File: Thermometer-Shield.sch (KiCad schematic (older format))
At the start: 33 parts, among them J1 CONN_01X04, J2 CONN_01X02, J3 CONN_01X02, J4 CONN_01X02, J5 CONN_01X02, SW1 SW_SPST, SW2 SW_SPST, SW3 SW_SPST, SW4 SW_SPST, U1 ULN2803A

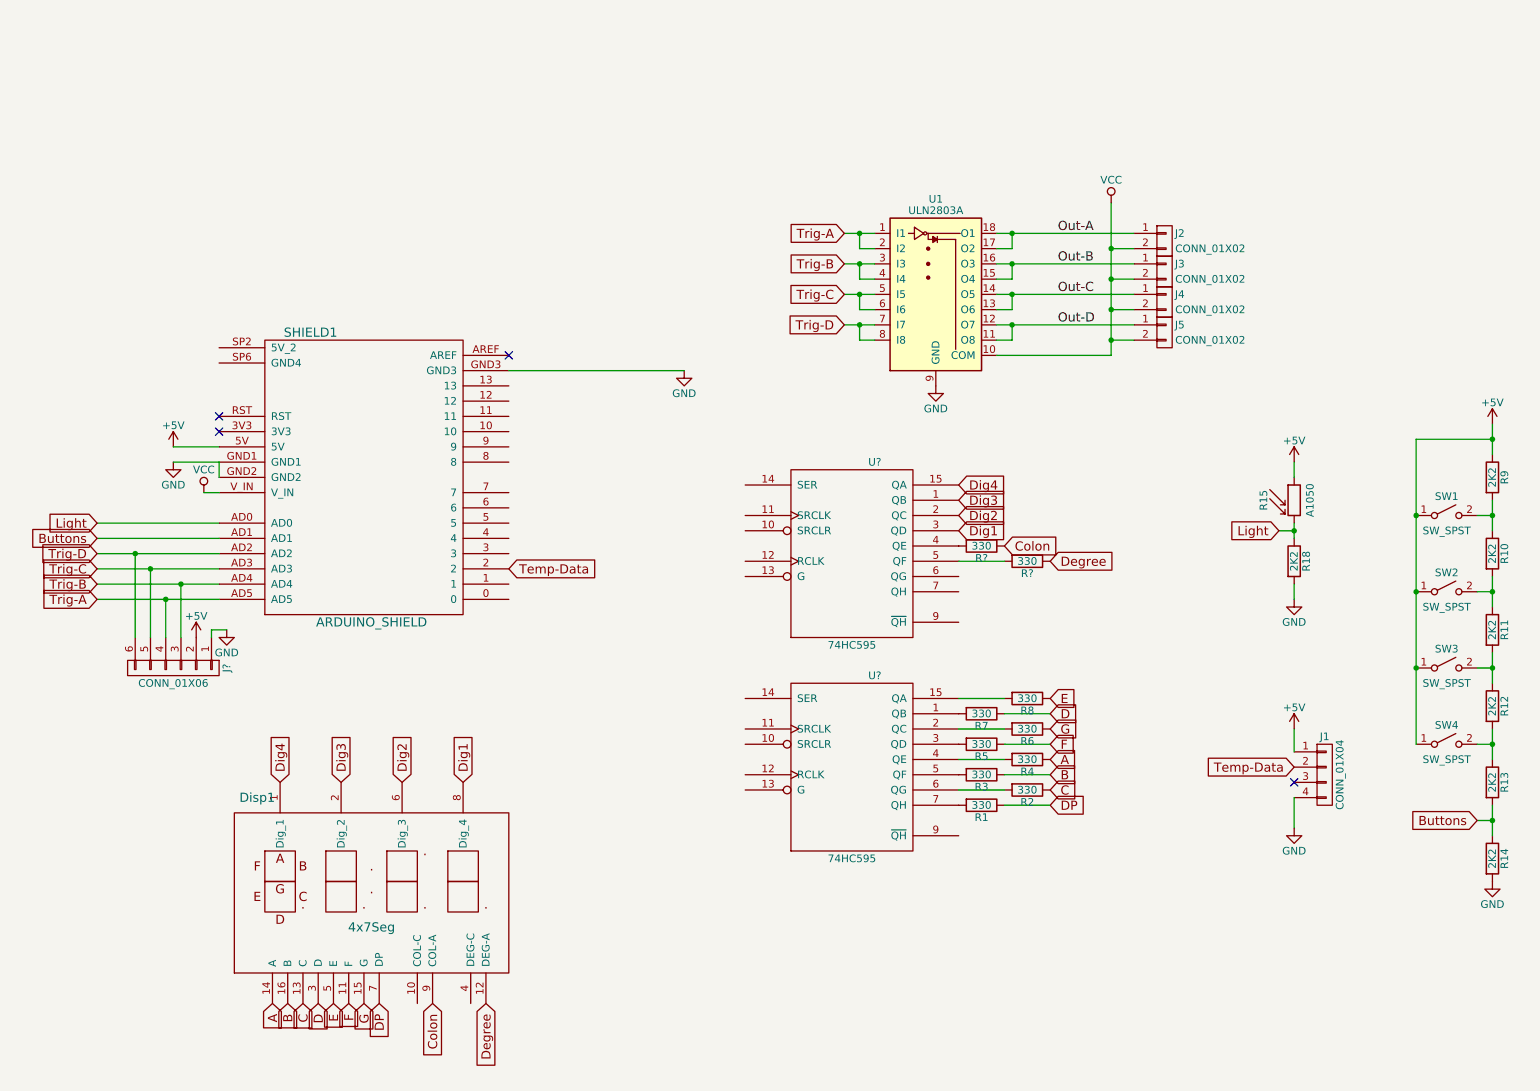
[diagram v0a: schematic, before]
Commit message: schematic nearly done. PCB started
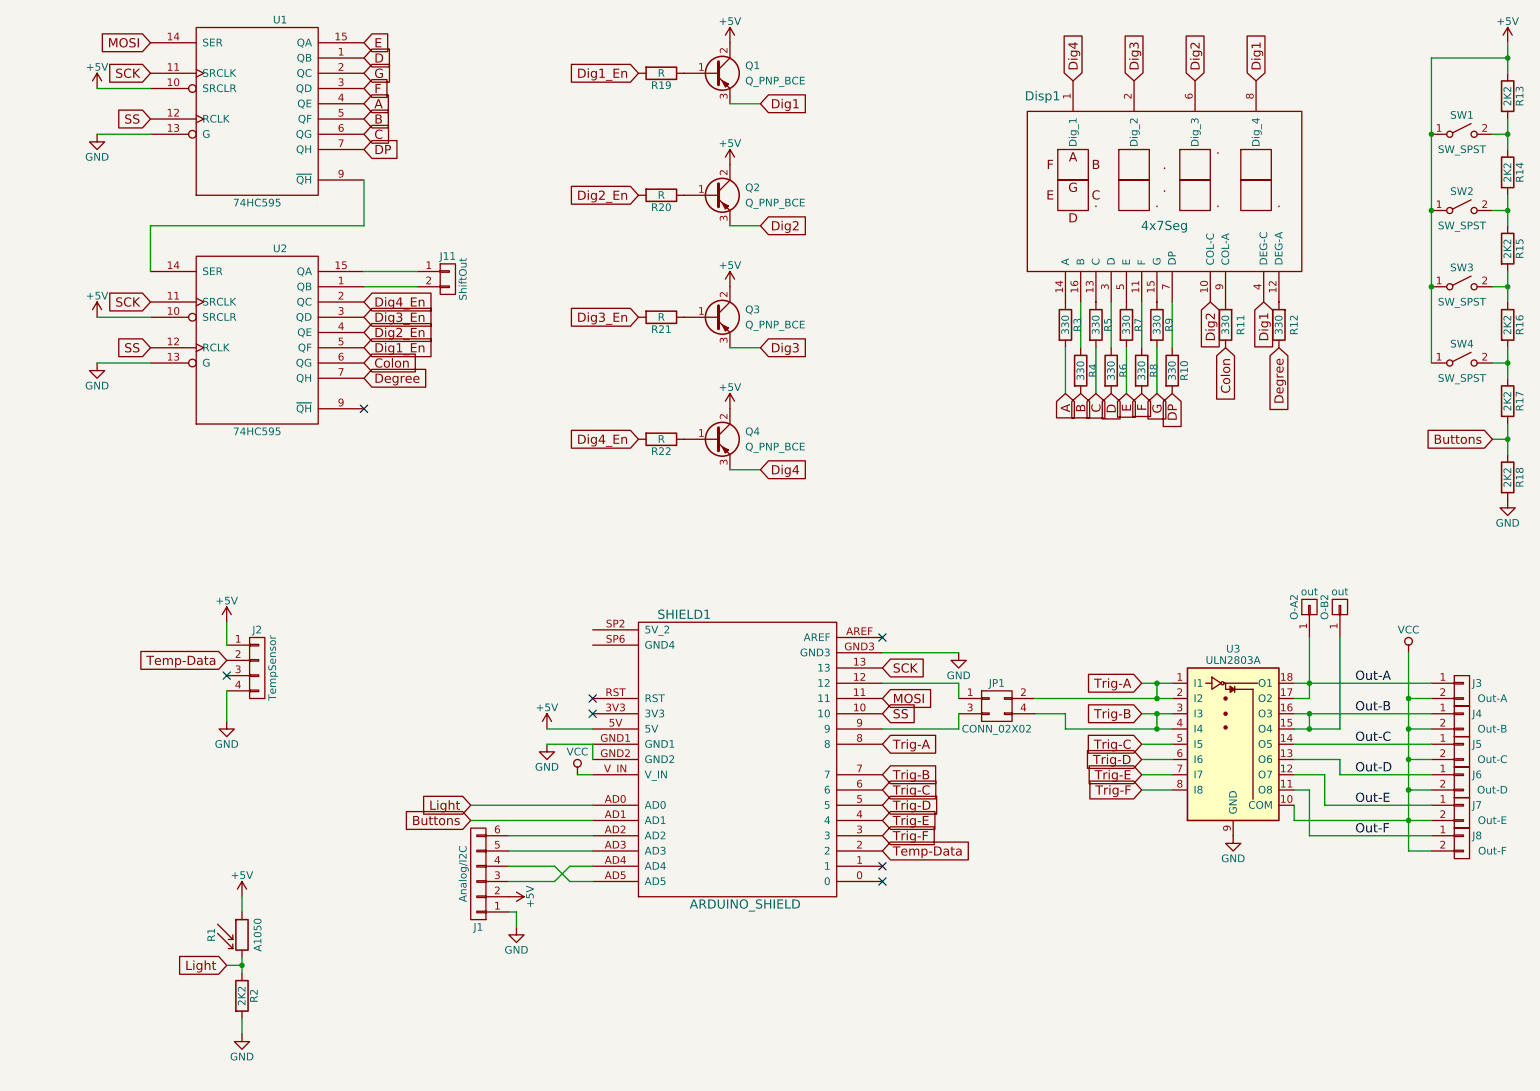
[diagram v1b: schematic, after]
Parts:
- added J11: ShiftOut, Pin_Headers:Pin_Header_Straight_1x02_Pitch2.54mm, symbol CONN_01X02
- added J7: Out-E, Connectors:AK300-2, symbol CONN_01X02
- added J8: Out-F, Connectors:AK300-2, symbol CONN_01X02
- added JP1: CONN_02X02, Pin_Headers:Pin_Header_Straight_2x02_Pitch2.54mm, symbol CONN_02X02
- added O-A2, O-B2: out, Connectors:1pin, symbol CONN_01X01
- added Q1, Q2, Q3, Q4: Q_PNP_BCE, TO_SOT_Packages_THT:TO-92_Inline_Narrow_Oval, symbol Q_PNP_BCE
- added R19, R20, R21, R22: R, Resistors_SMD:R_0805_HandSoldering, symbol R
- J1: renamed from J?; value CONN_01X06 -> Analog/I2C; footprint (none) -> Pin_Headers:Pin_Header_Straight_1x06_Pitch2.54mm
- J2: renamed from J1; value CONN_01X04 -> TempSensor
- J3: renamed from J2; value CONN_01X02 -> Out-A
- J4: renamed from J3; value CONN_01X02 -> Out-B
- J5: renamed from J4; value CONN_01X02 -> Out-C
- J6: renamed from J5; value CONN_01X02 -> Out-D
- R10: renamed from R1; footprint Resistors_SMD:R_0805_HandSoldering -> Resistors_SMD:R_0603_HandSoldering
- R11, R12: renamed from R?; footprint (none) -> Resistors_SMD:R_0603_HandSoldering
- R3: renamed from R8; footprint Resistors_SMD:R_0805_HandSoldering -> Resistors_SMD:R_0603_HandSoldering
- R4: renamed from R7; footprint Resistors_SMD:R_0805_HandSoldering -> Resistors_SMD:R_0603_HandSoldering
- R5: renamed from R6; footprint Resistors_SMD:R_0805_HandSoldering -> Resistors_SMD:R_0603_HandSoldering
- R6: renamed from R5; footprint Resistors_SMD:R_0805_HandSoldering -> Resistors_SMD:R_0603_HandSoldering
- R7: renamed from R4; footprint Resistors_SMD:R_0805_HandSoldering -> Resistors_SMD:R_0603_HandSoldering
- R8: renamed from R3; footprint Resistors_SMD:R_0805_HandSoldering -> Resistors_SMD:R_0603_HandSoldering
- R9: renamed from R2; footprint Resistors_SMD:R_0805_HandSoldering -> Resistors_SMD:R_0603_HandSoldering
- U1, U2: renamed from U?; footprint (none) -> Housings_SSOP:TSSOP-16_4.4x5mm_Pitch0.65mm
- renumbered R15 to R1, R9 to R13, R10 to R14, R11 to R15, R12 to R16, R13 to R17, R14 to R18, R18 to R2, U1 to U3
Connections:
- net +5V: now also U1.10 (SRCLR), U2.10 (SRCLR), Q1.2 (C), Q2.2 (C), Q3.2 (C), Q4.2 (C)
- net A: now also R3.2, U1.4 (QE); no longer Disp1.14 (A), R7.1
- net B: now also R4.2, U1.5 (QF); no longer Disp1.16 (B), R8.1
- net C: now also R5.2, U1.6 (QG); no longer Disp1.13 (C), R9.1
- net Colon: now also U2.6 (QG); no longer Disp1.9 (COL-A)
- net D: now also R6.2, U1.1 (QB); no longer Disp1.3 (D), R4.1
- net DP: now also R10.2, U1.7 (QH); no longer Disp1.7 (DP), R10.1
- net Degree: now also U2.7 (QH); no longer Disp1.12 (DEG-A)
- net Dig1: now also Disp1.4 (DEG-C), Q1.3 (E); no longer U2.3 (QD)
- net Dig2: now also Disp1.10 (COL-C), Q2.3 (E); no longer U2.2 (QC)
- net Dig3: now also Q3.3 (E); no longer U2.1 (QB)
- net Dig4: now also Q4.3 (E); no longer U2.15 (QA)
- net E: now also R7.2, U1.15 (QA); no longer Disp1.5 (E), R3.1
- net F: now also R8.2, U1.3 (QD); no longer Disp1.11 (F), R6.1
- net G: now also R9.2, U1.2 (QC); no longer Disp1.15 (G), R5.1
- net GND: now also U1.13 (G), U2.13 (G)
- net Out-A: now also O-A2.1 (P1)
- net Out-B: now also O-B2.1 (P1)
- net Out-C: no longer U3.13 (O6)
- net Out-D: now also U3.13 (O6); no longer U3.11 (O8), U3.12 (O7)
- net Trig-A: now also SHIELD1.8, JP1.2 (P2); no longer J1.4 (P4), SHIELD1.AD5
- net Trig-B: now also SHIELD1.7, JP1.4 (P4); no longer J1.3 (P3), SHIELD1.AD4
- net Trig-C: now also SHIELD1.6; no longer J1.5 (P5), SHIELD1.AD3, U3.6 (I6)
- net Trig-D: now also SHIELD1.5, U3.6 (I6); no longer J1.6 (P6), SHIELD1.AD2, U3.7 (I7), U3.8 (I8)
- net VCC: now also J7.2 (P2), J8.2 (P2)
- net SS: now reaches SHIELD1.10
- net SS: now also U1.12 (RCLK), U2.12 (RCLK)
- net MOSI: now reaches SHIELD1.11
- net MOSI: now also U1.14 (SER)
- net at SHIELD1.12: now also JP1.1 (P1)
- net SCK: now reaches SHIELD1.13
- net SCK: now also U1.11 (SRCLK), U2.11 (SRCLK)
- net Trig-F: now reaches SHIELD1.3
- net Trig-F: now also U3.8 (I8)
- net Trig-E: now reaches SHIELD1.4
- net Trig-E: now also U3.7 (I7)
- net at SHIELD1.9: now also JP1.3 (P3)
- net at U1.9 (~QH): now also U2.14 (SER)
- net at R11.2: now also Disp1.9 (COL-A); no longer U2.4 (QE)
- net at R12.2: now also Disp1.12 (DEG-A); no longer U2.5 (QF)
- new net: J1.6 (P6), SHIELD1.AD2
- new net: J1.5 (P5), SHIELD1.AD3
- new net: J1.3 (P3), SHIELD1.AD4
- new net: J1.4 (P4), SHIELD1.AD5
- new net: Disp1.7 (DP), R10.1
- new net: Disp1.15 (G), R9.1
- new net: Disp1.11 (F), R8.1
- new net: Disp1.5 (E), R7.1
- new net: Disp1.3 (D), R6.1
- new net: Disp1.13 (C), R5.1
- new net: Disp1.16 (B), R4.1
- new net: Disp1.14 (A), R3.1
- new net: J11.2 (P2), U2.1 (QB)
- new net: J11.1 (P1), U2.15 (QA)
- new net: Q1.1 (B), R19.1
- new net: Q2.1 (B), R20.1
- new net: Q3.1 (B), R21.1
- new net: Q4.1 (B), R22.1
- new net Dig1_En: R19.2, U2.5 (QF)
- new net Dig2_En: R20.2, U2.4 (QE)
- new net Dig3_En: R21.2, U2.3 (QD)
- new net Dig4_En: R22.2, U2.2 (QC)
- new net Out-E: J7.1 (P1), U3.12 (O7)
- new net Out-F: J8.1 (P1), U3.11 (O8)
- no-connect marks 4 -> 7
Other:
- moved on the sheet: Disp1, J1, J2, J3, J4, J5, J6, R1, R10, R11, R12, R13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
